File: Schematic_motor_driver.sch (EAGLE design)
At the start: 29 parts, among them Q2 IRF540, Q3 IRF540, Q4 IRF540, Q5 IRF540, U1 IR2104PBF, U2 IR2104PBF

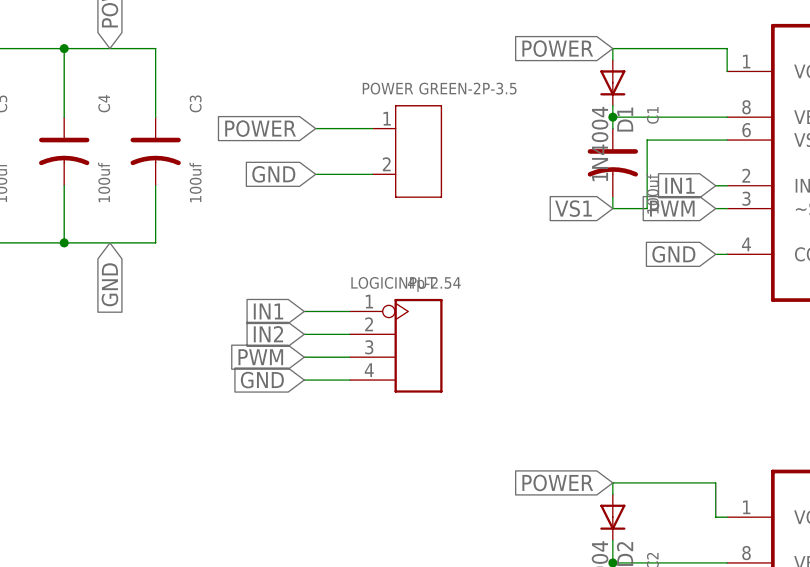
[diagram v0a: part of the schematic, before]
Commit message: final reviewed. Completed
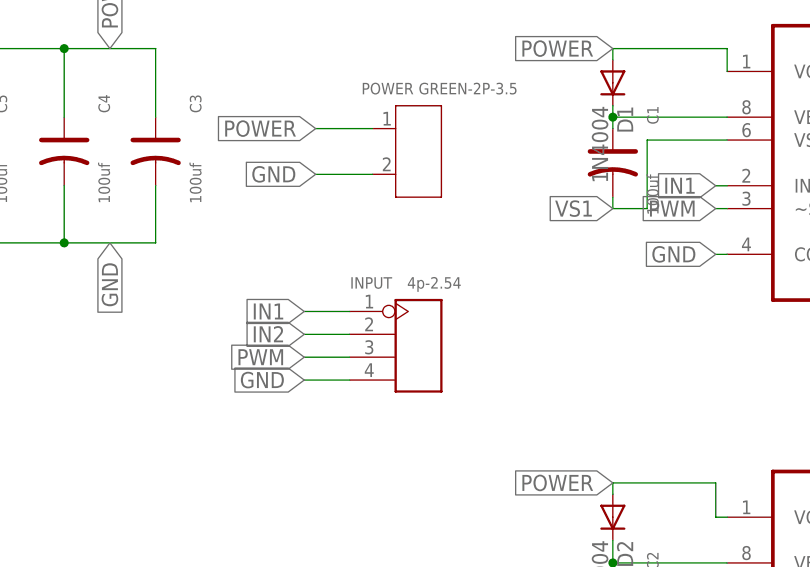
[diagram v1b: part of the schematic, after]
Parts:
- renumbered LOGICINPUT to INPUT
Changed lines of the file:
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@@
 <?xml version="1.0" encoding="utf-8"?>
 <!DOCTYPE eagle SYSTEM "eagle.dtd">
-<eagle version="7.6.0">
+<eagle version="7.2.0">
 <drawing>
 <settings>
@@
 <setting verticaltext="up"/>
 </settings>
-<grid distance="0.05" unitdist="inch" unit="inch" style="lines" multiple="1" display="no" altdistance="0.01" altunitdist="inch" altunit="inch"/>
+<grid distance="0.1" unitdist="inch" unit="inch" style="lines" multiple="1" display="no" altdistance="0.01" altunitdist="inch" altunit="inch"/>
 <layers>
 <layer number="1" name="Top" color="4" fill="1" visible="no" active="no"/>
@@
 <part name="U1" library="International_Rectifier_By_element14_Batch_1" deviceset="IR2104PBF" device=""/>
 <part name="U2" library="International_Rectifier_By_element14_Batch_1" deviceset="IR2104PBF" device=""/>
-<part name="LOGICINPUT" library="Seeed-Connector -2016" deviceset="DIP-BLACK-FEMALE-HEADER-VERT(4P-2.54)" device="" value="4p-2.54"/>
+<part name="INPUT" library="Seeed-Connector -2016" deviceset="DIP-BLACK-FEMALE-HEADER-VERT(4P-2.54)" device="" value="4p-2.54"/>
 <part name="POWER" library="Seeed-Connector -2016" deviceset="SCREW-TERMINAL-GREEN(2P-3.5)" device="" value="GREEN-2P-3.5"/>
 <part name="D1" library="adafruit" deviceset="1N4004" device=""/>
@@
 <instance part="U1" gate="A" x="53.34" y="88.9"/>
 <instance part="U2" gate="A" x="53.34" y="39.37"/>
-<instance part="LOGICINPUT" gate="G$1" x="1.27" y="66.04"/>
+<instance part="INPUT" gate="G$1" x="1.27" y="66.04"/>
 <instance part="POWER" gate="G$1" x="1.27" y="87.63"/>
 <instance part="D1" gate="1" x="22.86" y="95.25" rot="R270"/>
@@
 <net name="IN1" class="0">
 <segment>
-<pinref part="LOGICINPUT" gate="G$1" pin="P$1"/>
+<pinref part="INPUT" gate="G$1" pin="P$1"/>
 <wire x1="-6.35" y1="69.85" x2="-11.43" y2="69.85" width="0.1524" layer="91"/>
 <label x="-11.43" y="69.85" size="1.778" layer="95" rot="R180" xref="yes"/>
@@
 <net name="IN2" class="0">
 <segment>
-<pinref part="LOGICINPUT" gate="G$1" pin="P$2"/>
+<pinref part="INPUT" gate="G$1" pin="P$2"/>
 <wire x1="-6.35" y1="67.31" x2="-11.43" y2="67.31" width="0.1524" layer="91"/>
 <label x="-11.43" y="67.31" size="1.778" layer="95" rot="R180" xref="yes"/>
@@
 <net name="PWM" class="0">
 <segment>
-<pinref part="LOGICINPUT" gate="G$1" pin="P$3"/>
+<pinref part="INPUT" gate="G$1" pin="P$3"/>
 <wire x1="-11.43" y1="64.77" x2="-6.35" y2="64.77" width="0.1524" layer="91"/>
 <label x="-11.43" y="64.77" size="1.778" layer="95" rot="R180" xref="yes"/>
@@
 <net name="GND" class="0">
 <segment>
-<pinref part="LOGICINPUT" gate="G$1" pin="P$4"/>
+<pinref part="INPUT" gate="G$1" pin="P$4"/>
 <wire x1="-6.35" y1="62.23" x2="-11.43" y2="62.23" width="0.1524" layer="91"/>
 <label x="-11.43" y="62.23" size="1.778" layer="95" rot="R180" xref="yes"/>

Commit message: Revert "PCB Cosmetics"
This reverts commit 40f95e063b70cdd7ef0c66ddfb49b8478f35fe8d.
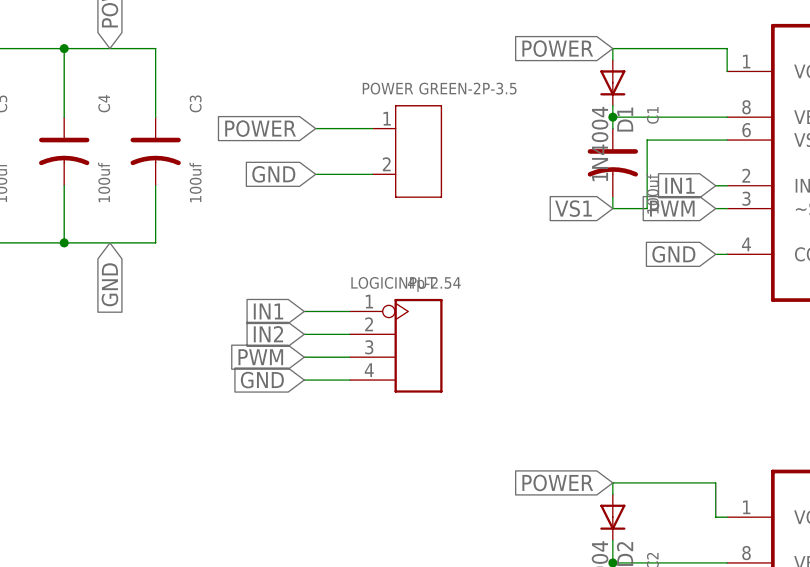
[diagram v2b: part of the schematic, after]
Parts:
- renumbered INPUT to LOGICINPUT
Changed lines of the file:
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@@
 <?xml version="1.0" encoding="utf-8"?>
 <!DOCTYPE eagle SYSTEM "eagle.dtd">
-<eagle version="7.2.0">
+<eagle version="7.6.0">
 <drawing>
 <settings>
@@
 <setting verticaltext="up"/>
 </settings>
-<grid distance="0.1" unitdist="inch" unit="inch" style="lines" multiple="1" display="no" altdistance="0.01" altunitdist="inch" altunit="inch"/>
+<grid distance="0.05" unitdist="inch" unit="inch" style="lines" multiple="1" display="no" altdistance="0.01" altunitdist="inch" altunit="inch"/>
 <layers>
 <layer number="1" name="Top" color="4" fill="1" visible="no" active="no"/>
@@
 <part name="U1" library="International_Rectifier_By_element14_Batch_1" deviceset="IR2104PBF" device=""/>
 <part name="U2" library="International_Rectifier_By_element14_Batch_1" deviceset="IR2104PBF" device=""/>
-<part name="INPUT" library="Seeed-Connector -2016" deviceset="DIP-BLACK-FEMALE-HEADER-VERT(4P-2.54)" device="" value="4p-2.54"/>
+<part name="LOGICINPUT" library="Seeed-Connector -2016" deviceset="DIP-BLACK-FEMALE-HEADER-VERT(4P-2.54)" device="" value="4p-2.54"/>
 <part name="POWER" library="Seeed-Connector -2016" deviceset="SCREW-TERMINAL-GREEN(2P-3.5)" device="" value="GREEN-2P-3.5"/>
 <part name="D1" library="adafruit" deviceset="1N4004" device=""/>
@@
 <instance part="U1" gate="A" x="53.34" y="88.9"/>
 <instance part="U2" gate="A" x="53.34" y="39.37"/>
-<instance part="INPUT" gate="G$1" x="1.27" y="66.04"/>
+<instance part="LOGICINPUT" gate="G$1" x="1.27" y="66.04"/>
 <instance part="POWER" gate="G$1" x="1.27" y="87.63"/>
 <instance part="D1" gate="1" x="22.86" y="95.25" rot="R270"/>
@@
 <net name="IN1" class="0">
 <segment>
-<pinref part="INPUT" gate="G$1" pin="P$1"/>
+<pinref part="LOGICINPUT" gate="G$1" pin="P$1"/>
 <wire x1="-6.35" y1="69.85" x2="-11.43" y2="69.85" width="0.1524" layer="91"/>
 <label x="-11.43" y="69.85" size="1.778" layer="95" rot="R180" xref="yes"/>
@@
 <net name="IN2" class="0">
 <segment>
-<pinref part="INPUT" gate="G$1" pin="P$2"/>
+<pinref part="LOGICINPUT" gate="G$1" pin="P$2"/>
 <wire x1="-6.35" y1="67.31" x2="-11.43" y2="67.31" width="0.1524" layer="91"/>
 <label x="-11.43" y="67.31" size="1.778" layer="95" rot="R180" xref="yes"/>
@@
 <net name="PWM" class="0">
 <segment>
-<pinref part="INPUT" gate="G$1" pin="P$3"/>
+<pinref part="LOGICINPUT" gate="G$1" pin="P$3"/>
 <wire x1="-11.43" y1="64.77" x2="-6.35" y2="64.77" width="0.1524" layer="91"/>
 <label x="-11.43" y="64.77" size="1.778" layer="95" rot="R180" xref="yes"/>
@@
 <net name="GND" class="0">
 <segment>
-<pinref part="INPUT" gate="G$1" pin="P$4"/>
+<pinref part="LOGICINPUT" gate="G$1" pin="P$4"/>
 <wire x1="-6.35" y1="62.23" x2="-11.43" y2="62.23" width="0.1524" layer="91"/>
 <label x="-11.43" y="62.23" size="1.778" layer="95" rot="R180" xref="yes"/>
